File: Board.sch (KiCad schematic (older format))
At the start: 17 parts, among them P1 Relay 1, P10 CONN_01X18, P11 CONN_01X18, P12 CONN_01X06, P2 Relay 2, P3 Relay 3, P4 Relay 4, P5 CONN_01X08, P6 CONN_01X08, P7 CONN_01X08, P8 CONN_01X08, P9 CONN_01X08

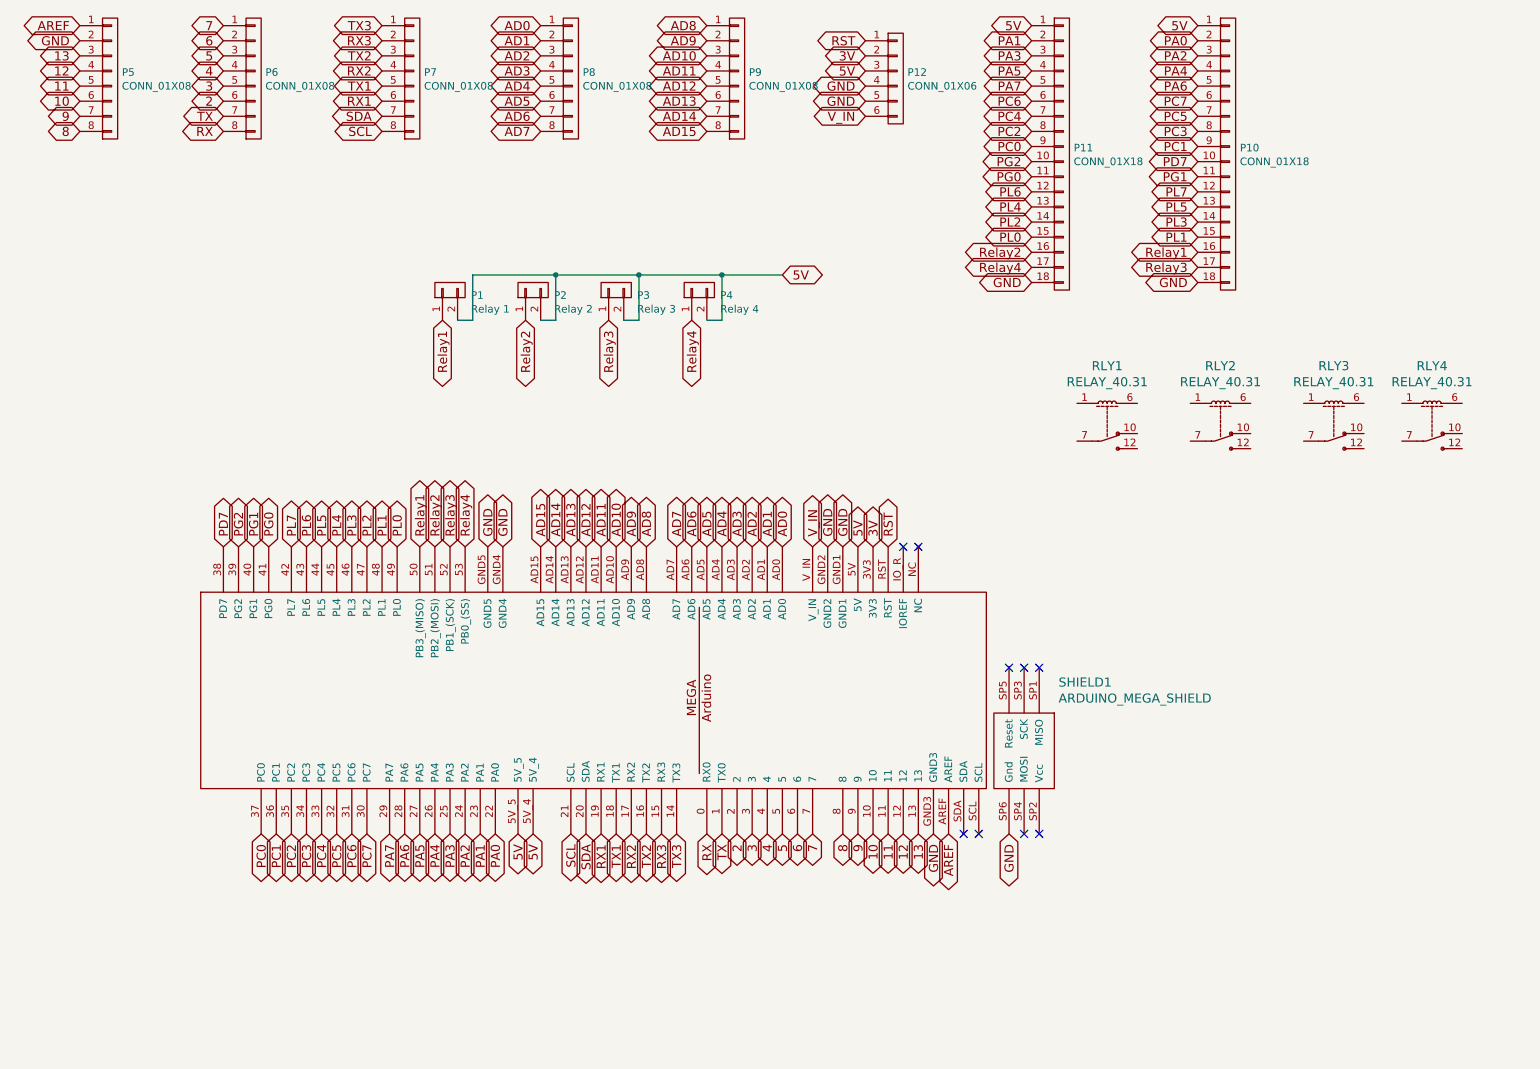
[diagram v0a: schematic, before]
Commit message: Cleaning Up Board
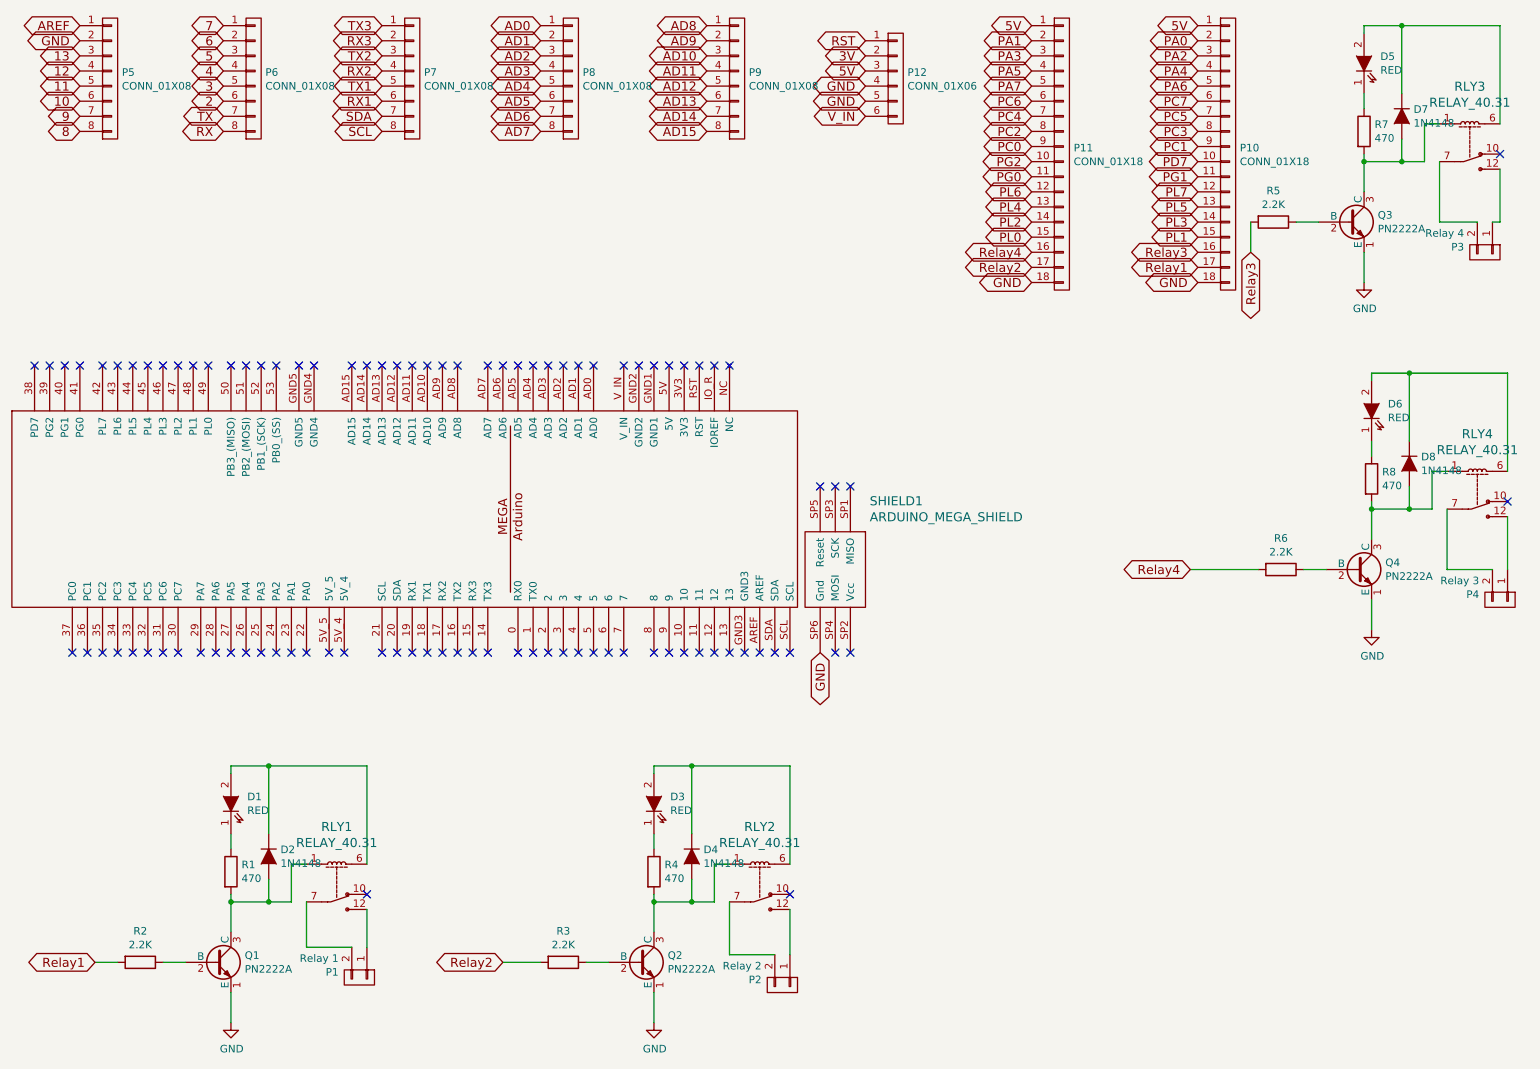
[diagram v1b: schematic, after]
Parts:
- added D1, D3, D5, D6: RED, LEDs:LED-3MM, symbol LED
- added D2, D4, D7, D8: 1N4148, Diodes_ThroughHole:Diode_DO-35_SOD27_Horizontal_RM10, symbol D
- added Q1, Q2, Q3, Q4: PN2222A, TO_SOT_Packages_THT:TO-92_Inline_Narrow_Oval, symbol PN2222A
- added R1, R4, R7, R8: 470, Resistors_ThroughHole:Resistor_Horizontal_RM7mm, symbol R
- added R2, R3, R5, R6: 2.2K, Resistors_ThroughHole:Resistor_Horizontal_RM7mm, symbol R
- P3: value Relay 3 -> Relay 4
- P4: value Relay 4 -> Relay 3
- RLY1: footprint Relays_THT:Relay_SPDS_OMRON-G6E -> Relays_ThroughHole:Relay_SPDS_OMRON-G6E
- RLY2, RLY3, RLY4: footprint Relays_THT:Relay_SPDS_OMRON-G6E -> Relays_ThroughHole:Relay_SPDS_OMRON-G6E; manf# (none) -> G6E-134P-US DC5
- SHIELD1: manf# (none) -> 2893
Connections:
- net 10: no longer SHIELD1.10
- net 11: no longer SHIELD1.11
- net 12: no longer SHIELD1.12
- net 13: no longer SHIELD1.13
- net 2: no longer SHIELD1.2
- net 3: no longer SHIELD1.3
- net 3V: no longer SHIELD1.3V3
- net 4: no longer SHIELD1.4
- net 5: no longer SHIELD1.5
- net 5V: no longer P1.2 (P2), P2.2 (P2), P3.2 (P2), P4.2 (P2), SHIELD1.5V, SHIELD1.5V_4, SHIELD1.5V_5
- net 6: no longer SHIELD1.6
- net 7: no longer SHIELD1.7
- net 8: no longer SHIELD1.8
- net 9: no longer SHIELD1.9
- net AD0: no longer SHIELD1.AD0
- net AD1: no longer SHIELD1.AD1
- net AD10: no longer SHIELD1.AD10
- net AD11: no longer SHIELD1.AD11
- net AD12: no longer SHIELD1.AD12
- net AD13: no longer SHIELD1.AD13
- net AD14: no longer SHIELD1.AD14
- net AD15: no longer SHIELD1.AD15
- net AD2: no longer SHIELD1.AD2
- net AD3: no longer SHIELD1.AD3
- net AD4: no longer SHIELD1.AD4
- net AD5: no longer SHIELD1.AD5
- net AD6: no longer SHIELD1.AD6
- net AD7: no longer SHIELD1.AD7
- net AD8: no longer SHIELD1.AD8
- net AD9: no longer SHIELD1.AD9
- net AREF: no longer SHIELD1.AREF
- net GND: now also Q1.1 (E), Q2.1 (E), Q3.1 (E), Q4.1 (E); no longer SHIELD1.GND1, SHIELD1.GND2, SHIELD1.GND3, SHIELD1.GND4, SHIELD1.GND5
- net PA0: no longer SHIELD1.22 (PA0)
- net PA1: no longer SHIELD1.23 (PA1)
- net PA2: no longer SHIELD1.24 (PA2)
- net PA3: no longer SHIELD1.25 (PA3)
- net PA4: no longer SHIELD1.26 (PA4)
- net PA5: no longer SHIELD1.27 (PA5)
- net PA6: no longer SHIELD1.28 (PA6)
- net PA7: no longer SHIELD1.29 (PA7)
- net PC0: no longer SHIELD1.37 (PC0)
- net PC1: no longer SHIELD1.36 (PC1)
- net PC2: no longer SHIELD1.35 (PC2)
- net PC3: no longer SHIELD1.34 (PC3)
- net PC4: no longer SHIELD1.33 (PC4)
- net PC5: no longer SHIELD1.32 (PC5)
- net PC6: no longer SHIELD1.31 (PC6)
- net PC7: no longer SHIELD1.30 (PC7)
- net PD7: no longer SHIELD1.38 (PD7)
- net PG0: no longer SHIELD1.41 (PG0)
- net PG1: no longer SHIELD1.40 (PG1)
- net PG2: no longer SHIELD1.39 (PG2)
- net PL0: no longer SHIELD1.49 (PL0)
- net PL1: no longer SHIELD1.48 (PL1)
- net PL2: no longer SHIELD1.47 (PL2)
- net PL3: no longer SHIELD1.46 (PL3)
- net PL4: no longer SHIELD1.45 (PL4)
- net PL5: no longer SHIELD1.44 (PL5)
- net PL6: no longer SHIELD1.43 (PL6)
- net PL7: no longer SHIELD1.42 (PL7)
- net RST: no longer SHIELD1.RST
- net RX: no longer SHIELD1.0 (RX0)
- net RX1: no longer SHIELD1.19 (RX1)
- net RX2: no longer SHIELD1.17 (RX2)
- net RX3: no longer SHIELD1.15 (RX3)
- net Relay1: now also P10.17 (P17), R2.2; no longer P1.1 (P1), P10.16 (P16), SHIELD1.50 (PB3_(MISO))
- net Relay2: now also P11.17 (P17), R3.2; no longer P11.16 (P16), P2.1 (P1), SHIELD1.51 (PB2_(MOSI))
- net Relay3: now also P10.16 (P16), R5.2; no longer P10.17 (P17), P3.1 (P1), SHIELD1.52 (PB1_(SCK))
- net Relay4: now also P11.16 (P16), R6.2; no longer P11.17 (P17), P4.1 (P1), SHIELD1.53 (PB0_(SS))
- net SCL: no longer SHIELD1.21 (SCL)
- net SDA: no longer SHIELD1.20 (SDA)
- net TX: no longer SHIELD1.1 (TX0)
- net TX1: no longer SHIELD1.18 (TX1)
- net TX2: no longer SHIELD1.16 (TX2)
- net TX3: no longer SHIELD1.14 (TX3)
- net V_IN: no longer SHIELD1.V_IN
- net at RLY1.1: now also D2.2 (A), Q1.3 (C), R1.2
- net at RLY1.12: now also P1.1 (P1)
- net at RLY1.6: now also D1.2 (A), D2.1 (K)
- net at RLY1.7: now also P1.2 (P2)
- net at RLY2.1: now also D4.2 (A), Q2.3 (C), R4.2
- net at RLY2.12: now also P2.1 (P1)
- net at RLY2.6: now also D3.2 (A), D4.1 (K)
- net at RLY2.7: now also P2.2 (P2)
- net at RLY3.1: now also D7.2 (A), Q3.3 (C), R7.2
- net at RLY3.12: now also P3.1 (P1)
- net at RLY3.6: now also D5.2 (A), D7.1 (K)
- net at RLY3.7: now also P3.2 (P2)
- net at RLY4.1: now also D8.2 (A), Q4.3 (C), R8.2
- net at RLY4.12: now also P4.1 (P1)
- net at RLY4.6: now also D6.2 (A), D8.1 (K)
- net at RLY4.7: now also P4.2 (P2)
- new net: D1.1 (K), R1.1
- new net: Q1.2 (B), R2.1
- new net: D3.1 (K), R4.1
- new net: Q2.2 (B), R3.1
- new net: D6.1 (K), R8.1
- new net: Q4.2 (B), R6.1
- new net: D5.1 (K), R7.1
- new net: Q3.2 (B), R5.1
- no-connect marks 9 -> 95
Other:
- moved on the sheet: P1, RLY1, SHIELD1
